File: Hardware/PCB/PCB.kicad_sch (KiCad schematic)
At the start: 167 parts, among them U1 ESP32-S3-DevKitC

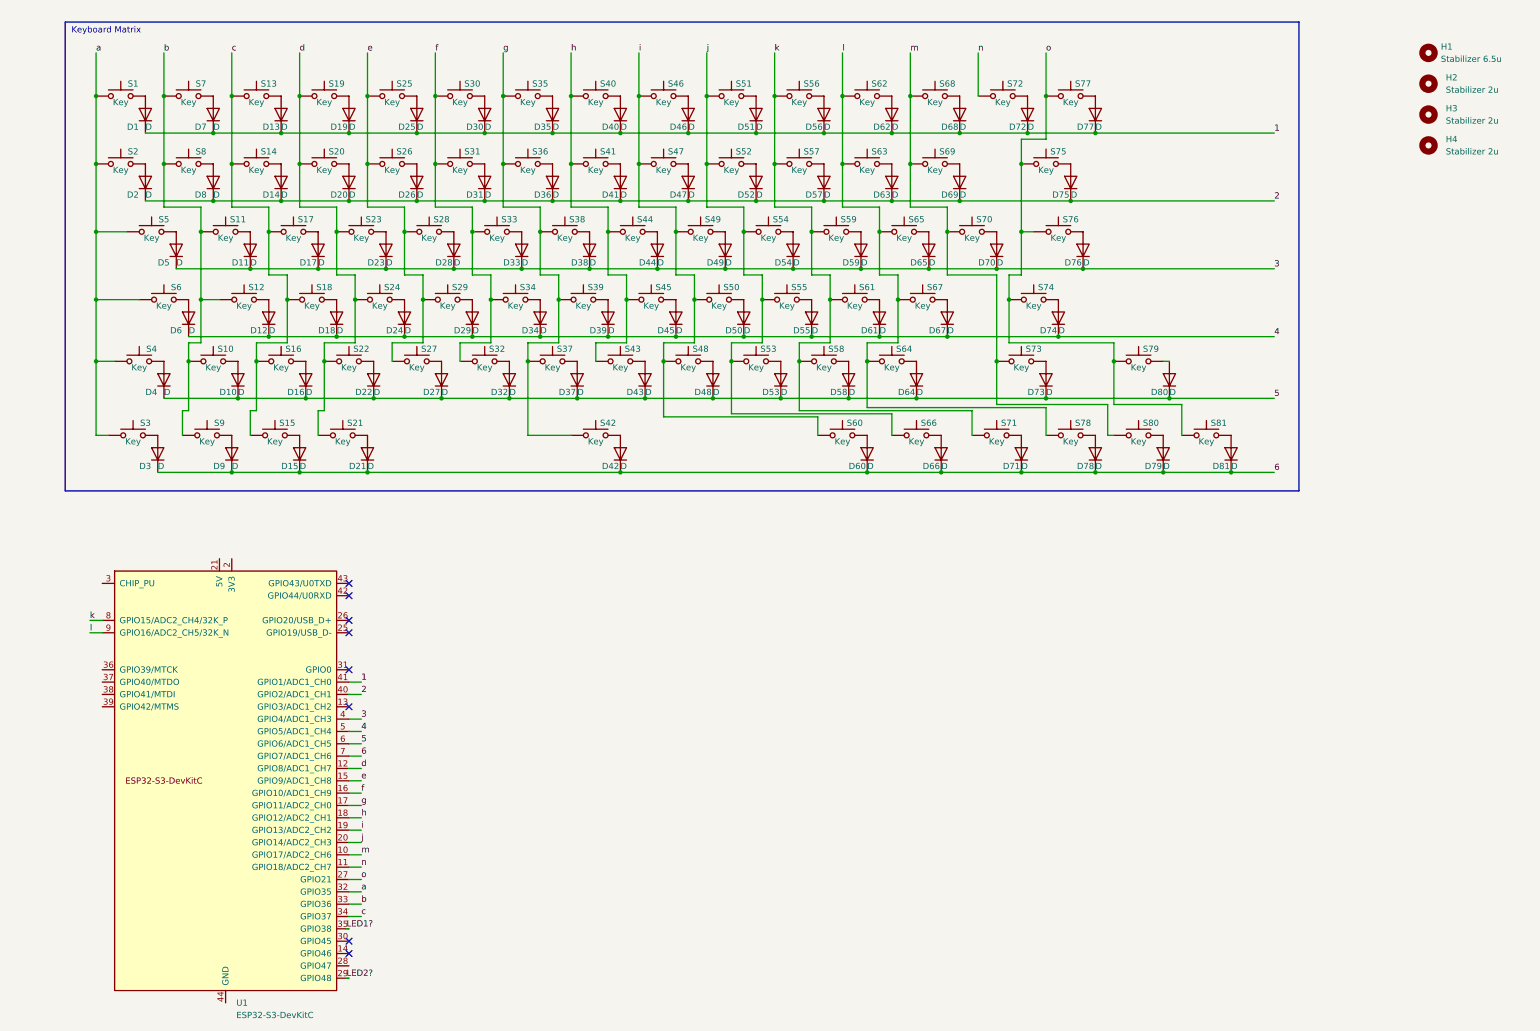
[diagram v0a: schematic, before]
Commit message: final hardware
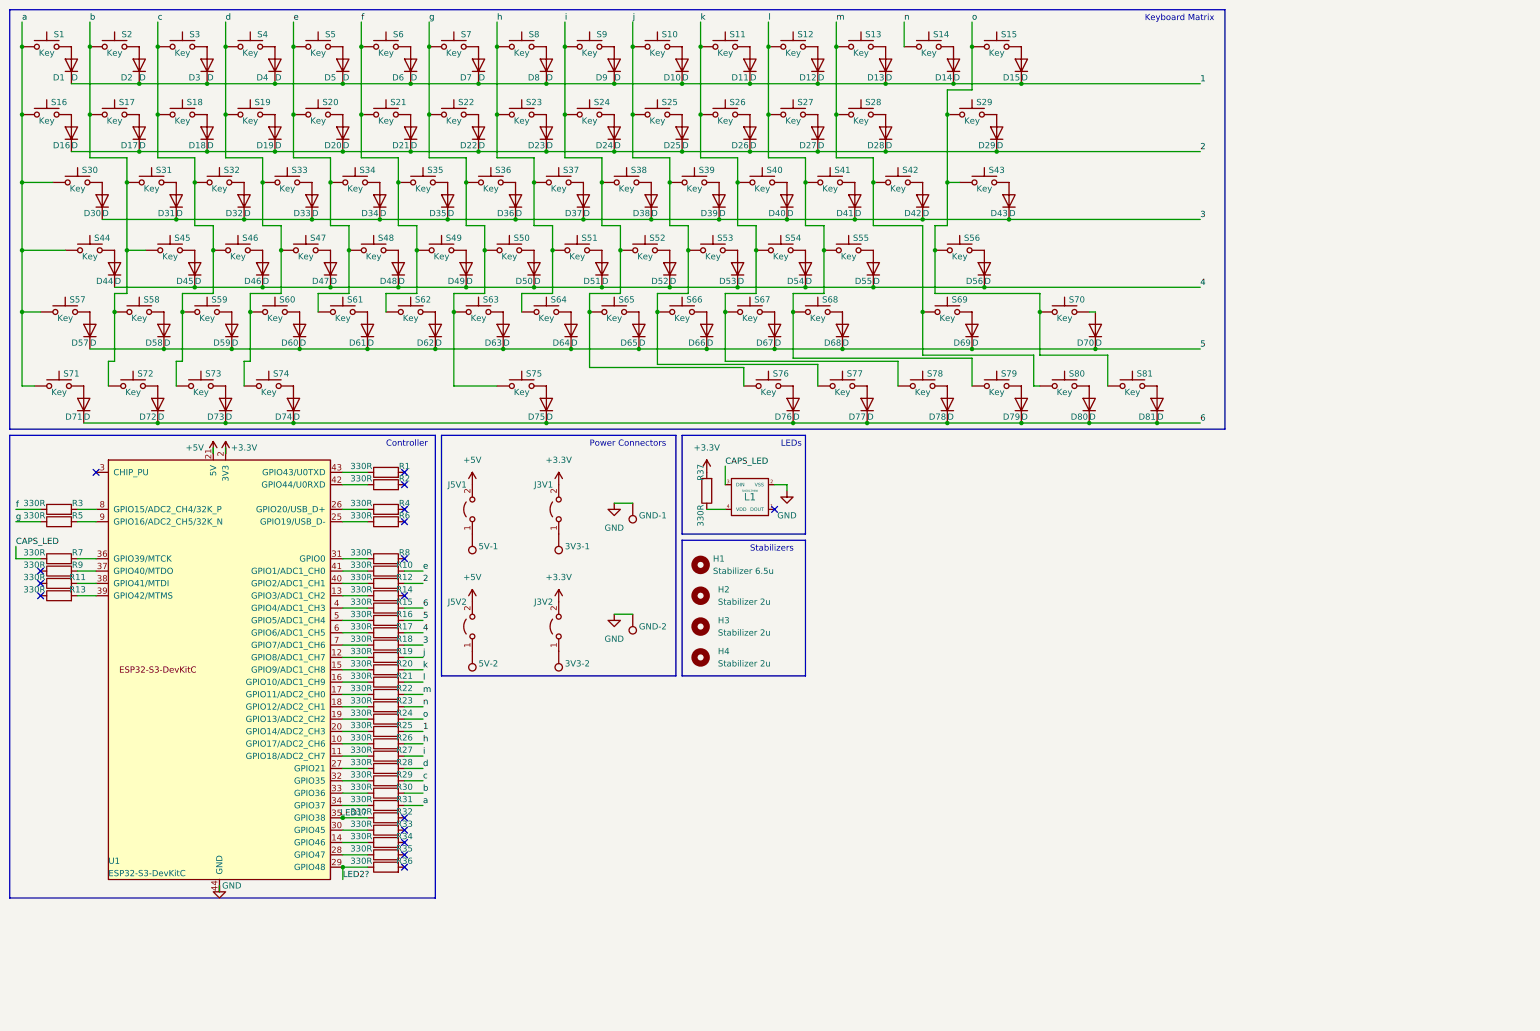
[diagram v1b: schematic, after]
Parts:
- added 3V3-1, 3V3-2, 5V-1, 5V-2, GND-1, GND-2: TestPoint, Connector_PinHeader_1.00mm:PinHeader_1x01_P1.00mm_Vertical, symbol Connector:TestPoint
- added J3V1, J3V2, J5V1, J5V2: Jumper_2_Open, Jumper:SolderJumper-2_P1.3mm_Open_TrianglePad1.0x1.5mm, symbol Jumper:Jumper_2_Open
- added L1: SK6812MINI, kbd:SK6812MINI_rev, symbol corne-classic-rescue:SK6812MINI-kbd
- added R1, R10, R11, R12, R13, R14, R15, R16, R17, R18, R19, R2, R20, R21, R22, R23, R24, R25, R26, R27, R28, R29, R3, R30, R31, R32, R33, R34, R35, R36, R37, R4, R5, R6, R7, R8, R9: 330R, Resistor_SMD:R_0603_1608Metric_Pad0.98x0.95mm_HandSolder, symbol Device:R
- renumbered D51 to D10, D56 to D11, D62 to D12, D68 to D13, D72 to D14, D77 to D15, D2 to D16, D8 to D17, D14 to D18, D20 to D19, D7 to D2, D26 to D20, D31 to D21, D36 to D22, D41 to D23, D47 to D24, D52 to D25, D57 to D26, D63 to D27, D69 to D28, D75 to D29, D13 to D3, D5 to D30, D11 to D31, D17 to D32, D23 to D33, D28 to D34, D33 to D35, D38 to D36, D44 to D37, D49 to D38, D54 to D39, D19 to D4, D59 to D40, D65 to D41, D70 to D42, D76 to D43, D6 to D44, D12 to D45, D18 to D46, D24 to D47, D29 to D48, D34 to D49, D25 to D5, D39 to D50, D45 to D51, D50 to D52, D55 to D53, D61 to D54, D67 to D55, D74 to D56, D4 to D57, D10 to D58, D16 to D59, D30 to D6, D22 to D60, D27 to D61, D32 to D62, D37 to D63, D43 to D64, D48 to D65, D53 to D66, D58 to D67, D64 to D68, D73 to D69, D35 to D7, D80 to D70, D3 to D71, D9 to D72, D15 to D73, D21 to D74, D42 to D75, D60 to D76, D66 to D77, D71 to D78, D78 to D79, D40 to D8, D79 to D80, D46 to D9, S51 to S10, S56 to S11, S62 to S12, S68 to S13, S72 to S14, S77 to S15, S2 to S16, S8 to S17, S14 to S18, S20 to S19, S7 to S2, S26 to S20, S31 to S21, S36 to S22, S41 to S23, S47 to S24, S52 to S25, S57 to S26, S63 to S27, S69 to S28, S75 to S29, S13 to S3, S5 to S30, S11 to S31, S17 to S32, S23 to S33, S28 to S34, S33 to S35, S38 to S36, S44 to S37, S49 to S38, S54 to S39, S19 to S4, S59 to S40, S65 to S41, S70 to S42, S76 to S43, S6 to S44, S12 to S45, S18 to S46, S24 to S47, S29 to S48, S34 to S49, S25 to S5, S39 to S50, S45 to S51, S50 to S52, S55 to S53, S61 to S54, S67 to S55, S74 to S56, S4 to S57, S10 to S58, S16 to S59, S30 to S6, S22 to S60, S27 to S61, S32 to S62, S37 to S63, S43 to S64, S48 to S65, S53 to S66, S58 to S67, S64 to S68, S73 to S69, S35 to S7, S79 to S70, S3 to S71, S9 to S72, S15 to S73, S21 to S74, S42 to S75, S60 to S76, S66 to S77, S71 to S78, S78 to S79, S40 to S8, S46 to S9
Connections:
- net 1: now also R25.2; no longer U1.41 (GPIO1/ADC1_CH0)
- net 2: now also R12.2; no longer U1.40 (GPIO2/ADC1_CH1)
- net 3: now also R18.2; no longer U1.4 (GPIO4/ADC1_CH3)
- net 4: now also R17.2; no longer U1.5 (GPIO5/ADC1_CH4)
- net 5: now also R16.2; no longer U1.6 (GPIO6/ADC1_CH5)
- net 6: now also R15.2; no longer U1.7 (GPIO7/ADC1_CH6)
- net LED1?: now also R32.1
- net LED2?: now also R36.1
- net a: now also R31.2; no longer U1.32 (GPIO35)
- net b: now also R30.2; no longer U1.33 (GPIO36)
- net c: now also R29.2; no longer U1.34 (GPIO37)
- net d: now also R28.2; no longer U1.12 (GPIO8/ADC1_CH7)
- net e: now also R10.2; no longer U1.15 (GPIO9/ADC1_CH8)
- net f: now also R3.1; no longer U1.16 (GPIO10/ADC1_CH9)
- net g: now also R5.1; no longer U1.17 (GPIO11/ADC2_CH0)
- net h: now also R26.2; no longer U1.18 (GPIO12/ADC2_CH1)
- net i: now also R27.2; no longer U1.19 (GPIO13/ADC2_CH2)
- net j: now also R19.2; no longer U1.20 (GPIO14/ADC2_CH3)
- net k: now also R20.2; no longer U1.8 (GPIO15/ADC2_CH4/32K_P)
- net l: now also R21.2; no longer U1.9 (GPIO16/ADC2_CH5/32K_N)
- net m: now also R22.2; no longer U1.10 (GPIO17/ADC2_CH6)
- net n: now also R23.2; no longer U1.11 (GPIO18/ADC2_CH7)
- net o: now also R24.2; no longer U1.27 (GPIO21)
- net +3.3V: now reaches U1.1 (3V3), U1.2 (3V3)
- net +3.3V: now also J3V1.2 (B), J3V2.2 (B), R37.2
- net at U1.13 (GPIO3/ADC1_CH2): now also R14.1
- net at U1.14 (GPIO46): now also R34.1
- net +5V: now reaches U1.21 (5V)
- net +5V: now also J5V1.2 (B), J5V2.2 (B)
- net GND: now reaches U1.22 (GND), U1.23 (GND), U1.24 (GND), U1.44 (GND)
- net GND: now also GND-1.1, GND-2.1, L1.2 (VSS)
- net at U1.25 (GPIO19/USB_D-): now also R6.1
- net at U1.26 (GPIO20/USB_D+): now also R4.1
- net at U1.28 (GPIO47): now also R35.1
- net at U1.30 (GPIO45): now also R33.1
- net at U1.31 (GPIO0): now also R8.1
- net at U1.36 (GPIO39/MTCK): now also R7.2
- net at U1.37 (GPIO40/MTDO): now also R9.2
- net at U1.38 (GPIO41/MTDI): now also R11.2
- net at U1.39 (GPIO42/MTMS): now also R13.2
- net at U1.42 (GPIO44/U0RXD): now also R2.1
- net at U1.43 (GPIO43/U0TXD): now also R1.1
- new net: L1.4 (VDD), R37.1
- new net: R30.1, U1.33 (GPIO36)
- new net: 5V-2.1, J5V2.1 (A)
- new net: 3V3-1.1, J3V1.1 (A)
- new net: R3.2, U1.8 (GPIO15/ADC2_CH4/32K_P)
- new net: 3V3-2.1, J3V2.1 (A)
- new net: R23.1, U1.18 (GPIO12/ADC2_CH1)
- new net: R29.1, U1.32 (GPIO35)
- new net: R15.1, U1.4 (GPIO4/ADC1_CH3)
- new net: R25.1, U1.20 (GPIO14/ADC2_CH3)
- new net: R27.1, U1.11 (GPIO18/ADC2_CH7)
- new net: R12.1, U1.40 (GPIO2/ADC1_CH1)
- new net: R19.1, U1.12 (GPIO8/ADC1_CH7)
- new net: R28.1, U1.27 (GPIO21)
- new net: R26.1, U1.10 (GPIO17/ADC2_CH6)
- new net: R20.1, U1.15 (GPIO9/ADC1_CH8)
- new net: R21.1, U1.16 (GPIO10/ADC1_CH9)
- new net: R22.1, U1.17 (GPIO11/ADC2_CH0)
- new net: R24.1, U1.19 (GPIO13/ADC2_CH2)
- new net: R31.1, U1.34 (GPIO37)
- new net: R10.1, U1.41 (GPIO1/ADC1_CH0)
- new net: R16.1, U1.5 (GPIO5/ADC1_CH4)
- new net: R17.1, U1.6 (GPIO6/ADC1_CH5)
- new net: R18.1, U1.7 (GPIO7/ADC1_CH6)
- new net: R5.2, U1.9 (GPIO16/ADC2_CH5/32K_N)
- new net: 5V-1.1, J5V1.1 (A)
- new net CAPS_LED: L1.3 (DIN), R7.1
- no-connect marks 8 -> 16
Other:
- note added: "Controller"
- note added: "LEDs"
- note added: "Power Connectors"
- note added: "Stabilizers"
- moved on the sheet: D1, D10, D11, D12, D13, D14, D15, D16, D17, D18, D19, D2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
